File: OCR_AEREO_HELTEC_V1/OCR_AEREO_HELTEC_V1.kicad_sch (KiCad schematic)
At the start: 30 parts, among them J1 Conn_01x04_Socket, J10 Conn_01x02_Pin, J11 Conn_01x02_Pin, J12 Conn_01x08_Socket, J13 Conn_01x04_Socket, J14 MODULO SD, J15 Conn_01x03_Pin, J16 Conn_01x04_Socket, J17 Screw_Terminal_01x03, J18 Screw_Terminal_01x03, J19 BIOSHUT, J2 Conn_01x04_Socket, J3 Conn_01x18_Pin, J4 Conn_01x02_Pin, J5 Conn_01x02_Pin, J6 OCR, J7 BATERÍA, J8 Conn_01x02_Pin, J9 Conn_01x02_Pin, U2 MAX3232

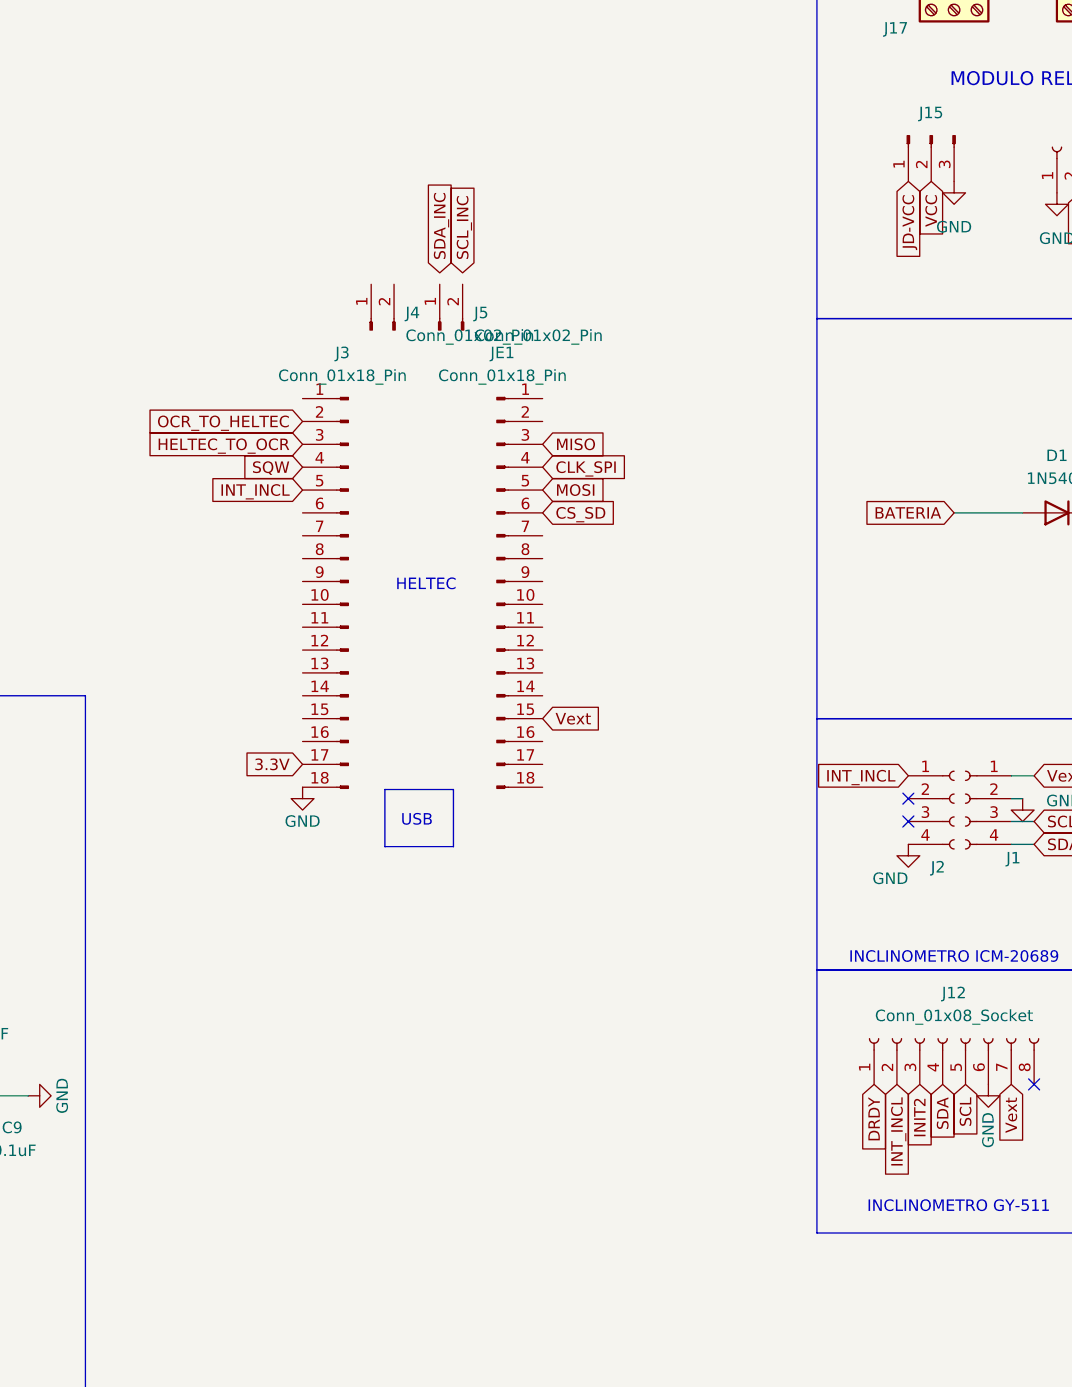
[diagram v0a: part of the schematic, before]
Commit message: actualizacion V2
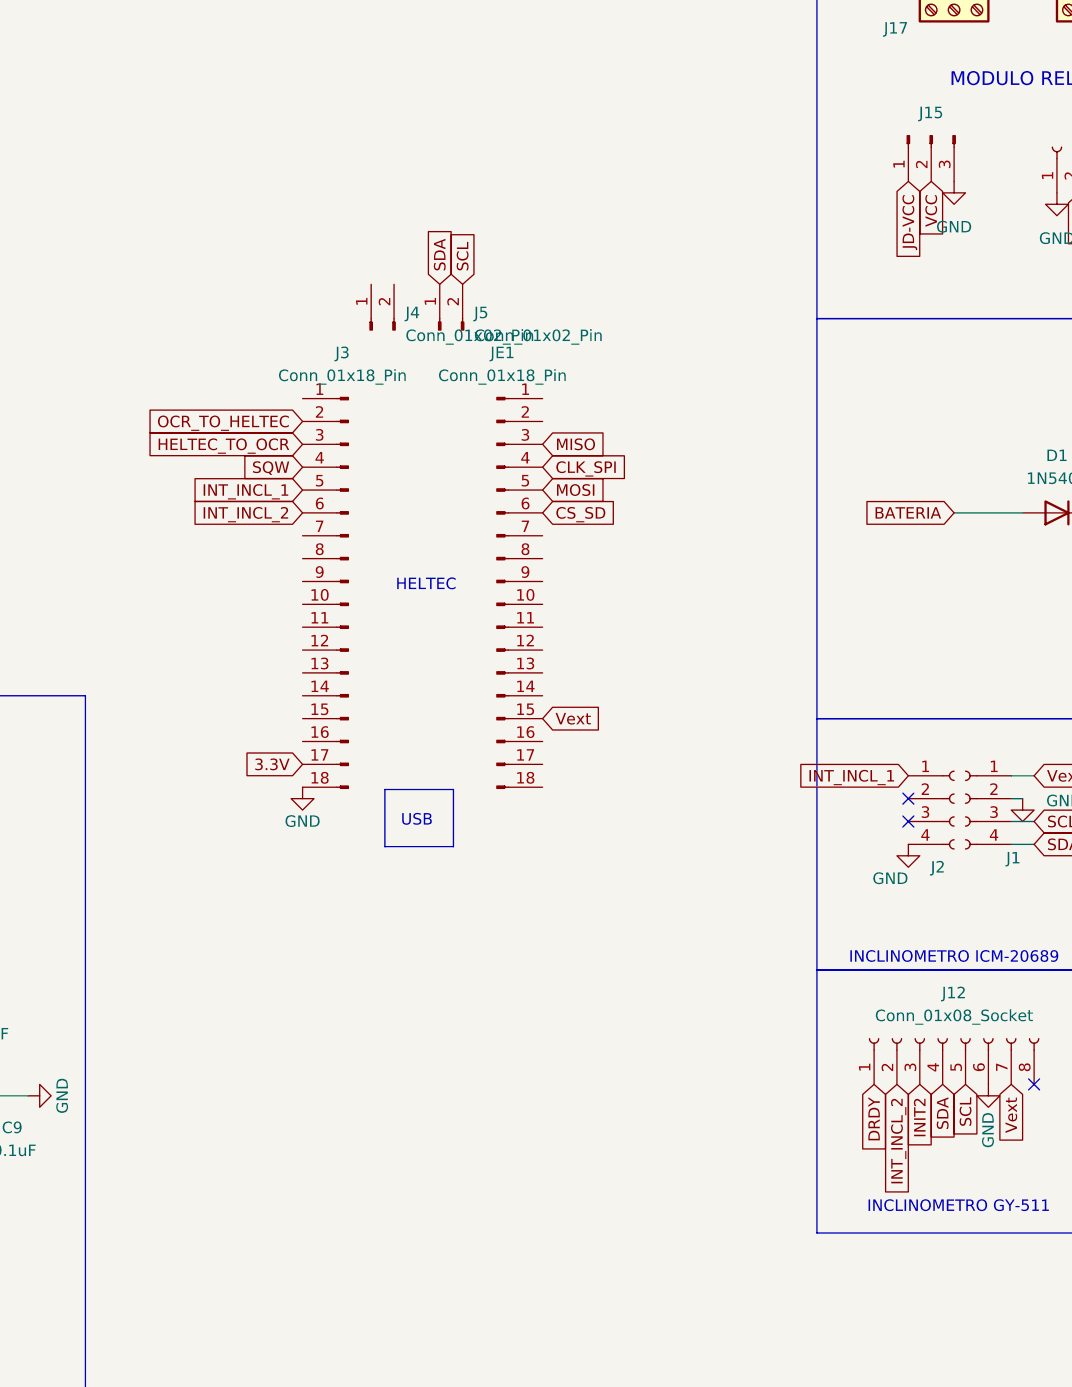
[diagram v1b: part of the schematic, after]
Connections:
- net SCL: now also J5.2 (Pin_2)
- net SDA: now also J5.1 (Pin_1)
- net INT_INCL_2: now reaches J3.6 (Pin_6)
- net INT_INCL_2: now also J12.2 (Pin_2)
- net INT_INCL renamed INT_INCL_1
- net INT_INCL_1: no longer J12.2 (Pin_2)
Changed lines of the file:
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@@
+		)
+	)
+	(global_label "INT_INCL_2"
+		(shape input)
+		(at 121.92 85.09 180)
+		(fields_autoplaced yes)
+		(effects
+			(font
+				(size 1.27 1.27)
+			)
+			(justify right)
+		)
+		(property "Intersheetrefs" "${INTERSHEET_REFS}"
+			(at 108.6538 85.09 0)
+			(hide yes)
+			(show_name no)
+			(do_not_autoplace no)
+			(effects
+				(font
+					(size 1.27 1.27)
+				)
+				(justify right)
+			)
 		)
 	)
@@
 		)
 	)
-	(global_label "SCL_INC"
-		(shape input)
-		(at 139.7 58.42 90)
-		(fields_autoplaced yes)
-		(effects
-			(font
-				(size 1.27 1.27)
-			)
-			(justify left)
-		)
-		(property "Intersheetrefs" "${INTERSHEET_REFS}"
-			(at 139.7 47.7543 90)
-			(hide yes)
-			(show_name no)
-			(do_not_autoplace no)
-			(effects
-				(font
-					(size 1.27 1.27)
-				)
-				(justify left)
-			)
-		)
-	)
 	(global_label "SCL"
 		(shape input)
+		(at 139.7 59.69 90)
+		(fields_autoplaced yes)
+		(effects
+			(font
+				(size 1.27 1.27)
+			)
+			(justify left)
+		)
+		(property "Intersheetrefs" "${INTERSHEET_REFS}"
+			(at 139.7 53.1972 90)
+			(hide yes)
+			(show_name no)
+			(do_not_autoplace no)
+			(effects
+				(font
+					(size 1.27 1.27)
+				)
+				(justify left)
+			)
+		)
+	)
+	(global_label "SCL"
+		(shape input)
 		(at 218.44 124.46 90)
 		(fields_autoplaced yes)
@@
 		)
 	)
-	(global_label "INT_INCL"
+	(global_label "INT_INCL_2"
 		(shape input)
 		(at 187.96 148.59 270)
@@
 		)
 		(property "Intersheetrefs" "${INTERSHEET_REFS}"
-			(at 187.96 159.6791 90)
+			(at 187.96 161.8562 90)
 			(hide yes)
 			(show_name no)
@@
 		)
 	)
-	(global_label "SDA_INC"
-		(shape input)
-		(at 137.16 58.42 90)
-		(fields_autoplaced yes)
-		(effects
-			(font
-				(size 1.27 1.27)
-			)
-			(justify left)
-		)
-		(property "Intersheetrefs" "${INTERSHEET_REFS}"
-			(at 137.16 47.6938 90)
+	(global_label "SDA"
+		(shape input)
+		(at 137.16 59.69 90)
+		(fields_autoplaced yes)
+		(effects
+			(font
+				(size 1.27 1.27)
+			)
+			(justify left)
+		)
+		(property "Intersheetrefs" "${INTERSHEET_REFS}"
+			(at 137.16 53.1367 90)
 			(hide yes)
 			(show_name no)
@@
 		)
 	)
-	(global_label "INT_INCL"
+	(global_label "INT_INCL_1"
 		(shape input)
 		(at 121.92 82.55 180)
@@
 		)
 		(property "Intersheetrefs" "${INTERSHEET_REFS}"
-			(at 110.8309 82.55 0)
-			(hide yes)
-			(show_name no)
-			(do_not_autoplace no)
-			(effects
-				(font
-					(size 1.27 1.27)
-				)
-				(justify right)
-			)
-		)
-	)
-	(global_label "INT_INCL"
+			(at 108.6538 82.55 0)
+			(hide yes)
+			(show_name no)
+			(do_not_autoplace no)
+			(effects
+				(font
+					(size 1.27 1.27)
+				)
+				(justify right)
+			)
+		)
+	)
+	(global_label "INT_INCL_1"
 		(shape input)
 		(at 189.23 114.3 180)
@@
 		)
 		(property "Intersheetrefs" "${INTERSHEET_REFS}"
-			(at 178.1409 114.3 0)
-			(hide yes)
-			(show_name no)
+			(at 175.9638 114.3 0)
+			(hide yes)
+			(show_name no)
